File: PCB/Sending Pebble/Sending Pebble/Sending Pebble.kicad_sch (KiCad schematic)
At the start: 46 parts, among them J1 USB_C_Receptacle_USB2.0_16P, J2 Conn_01x02_Socket, J3 u.Fl, J4 SMA, J5 Conn_01x02_Socket, Q1 IRLML0030, SW2 RESET, SW3 BOOT, U1 LoRa-E5, U3 MAX-M10S, U4 BMP390, U5 AZ1117CH2-3.3, U6 CP2102N-Axx-xQFN24, U7 BQ24072RGT

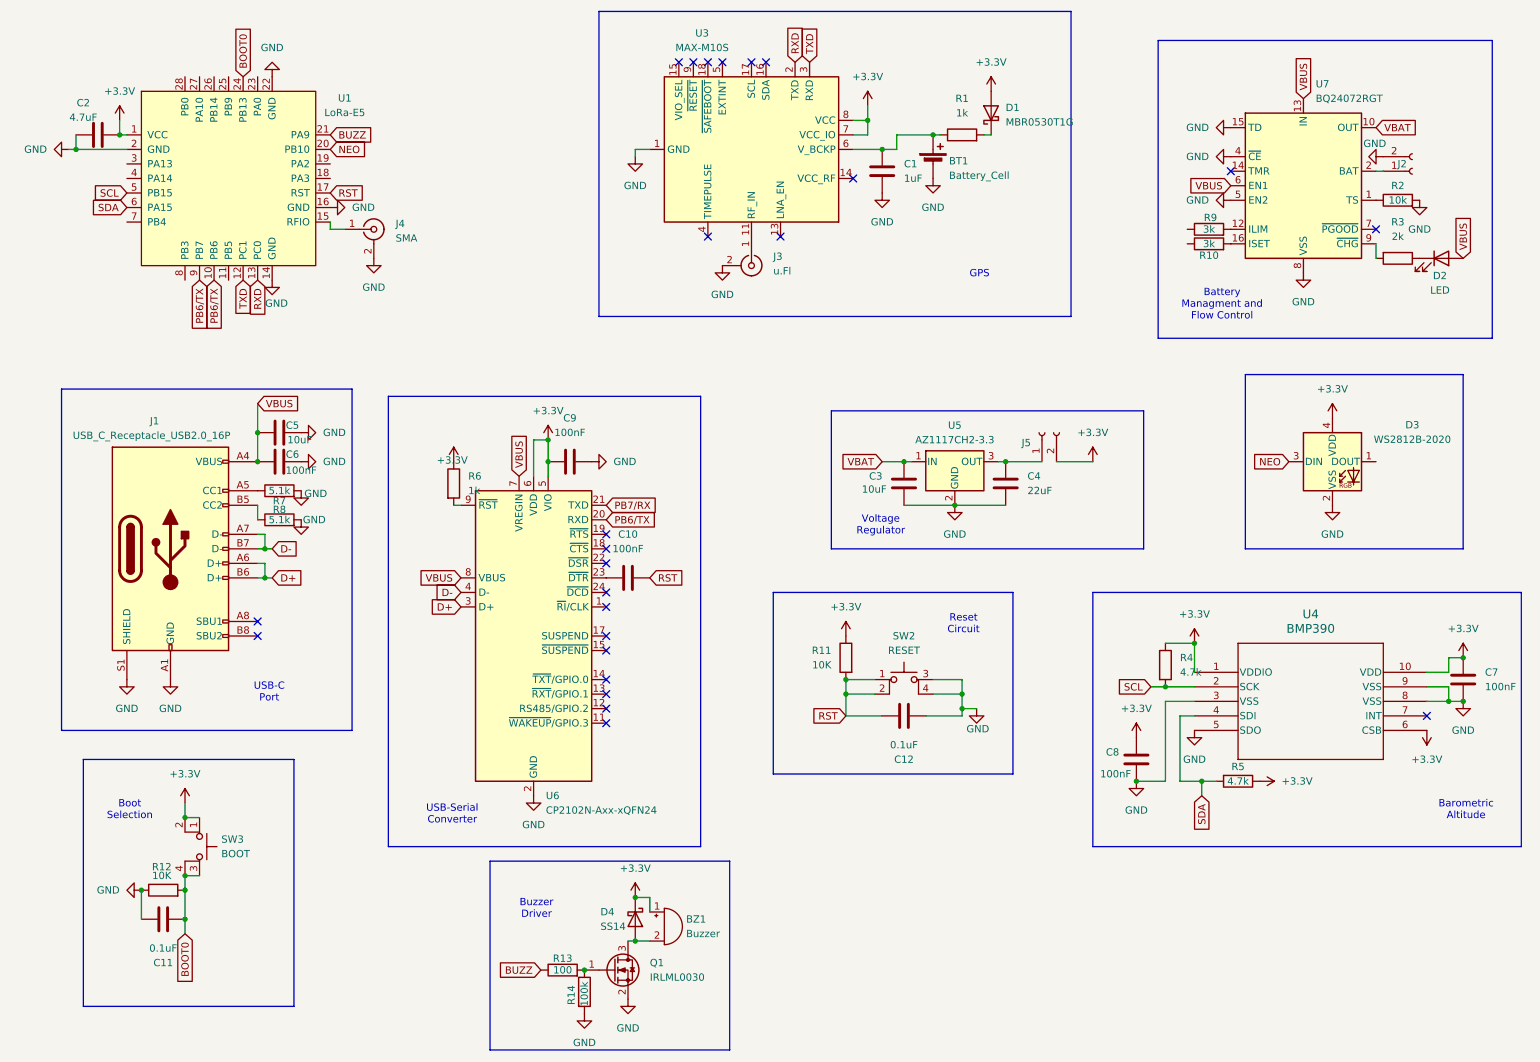
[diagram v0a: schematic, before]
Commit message: Started Layout, Added DRC
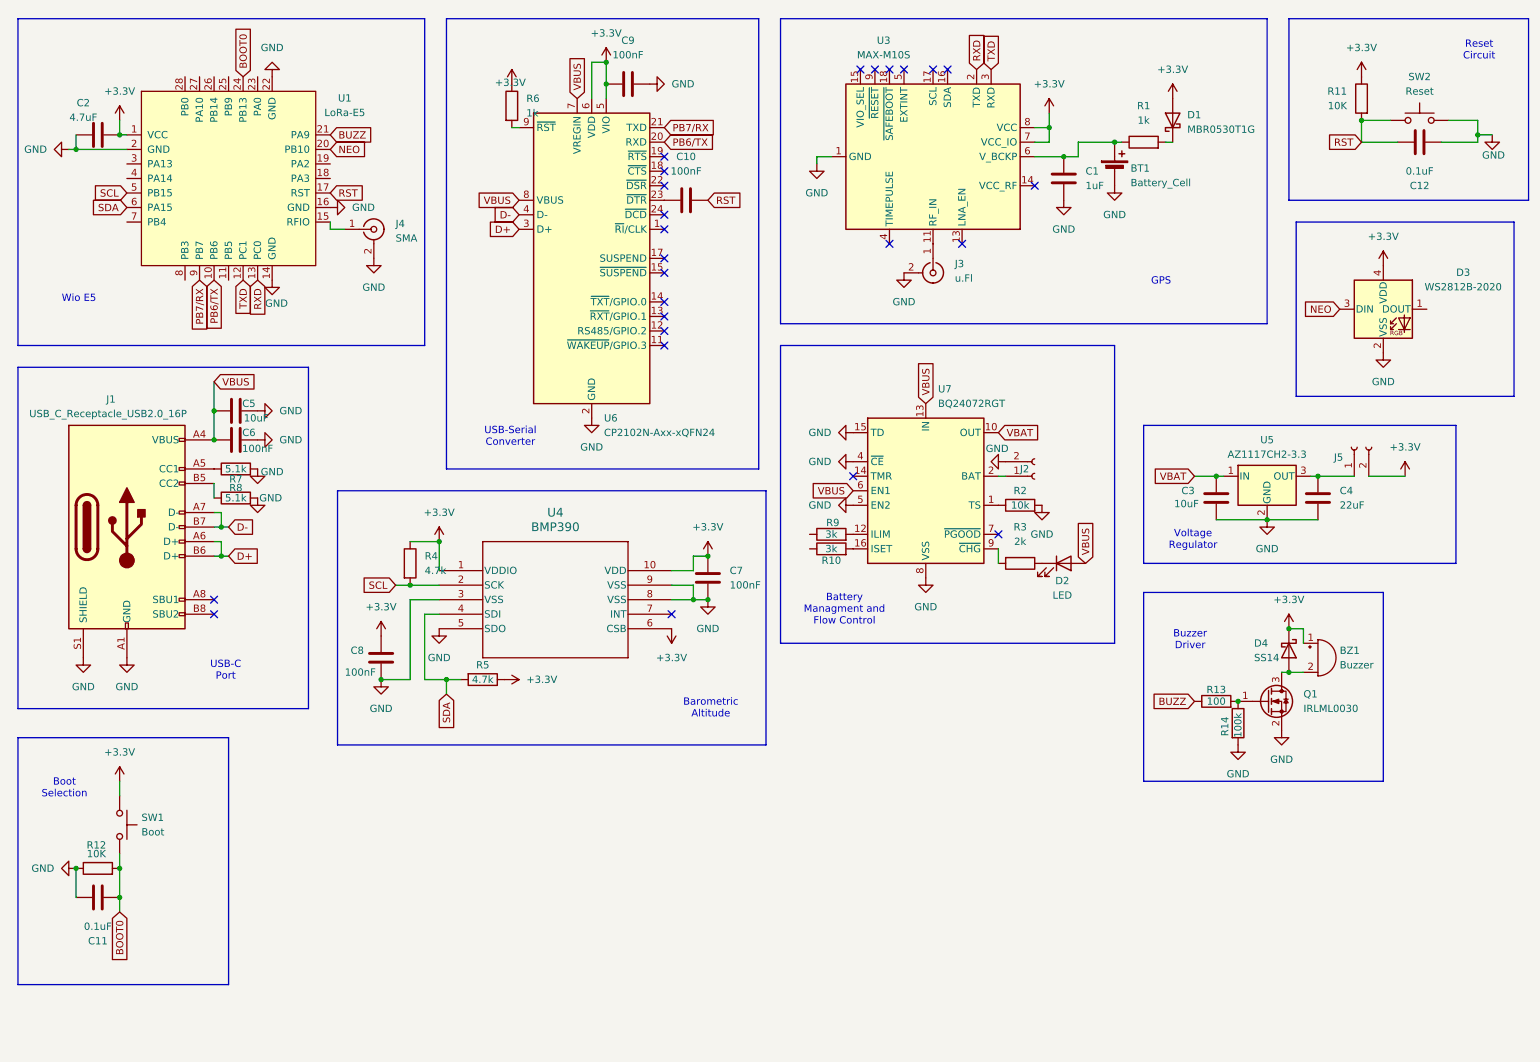
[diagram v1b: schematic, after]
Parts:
- removed SW2: RESET, Button_Switch_SMD:SW_SPST_PTS810, symbol Switch:SW_MEC_5E
- removed SW3: BOOT, Button_Switch_SMD:SW_SPST_PTS810, symbol Switch:SW_MEC_5E
- added SW1: Boot, Button_Switch_SMD:SW_SPST_PTS810, symbol Switch:SW_Push
- added SW2: Reset, Button_Switch_SMD:SW_SPST_PTS810, symbol Switch:SW_Push
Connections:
- net +3.3V: now also SW1.1
- net BOOT0: now also SW1.2
- net GND: now also SW2.2
- net PB6/TX: no longer U1.9 (PB7)
- net PB7/RX: now also U1.9 (PB7)
- net RST: now also SW2.1
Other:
- note added: "Wio E5"
- title: (none) -> Sending Pebble v1
- moved on the sheet: BT1, BZ1, C1, C10, C11, C12, C3, C4, C5, C6, C7, C8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
